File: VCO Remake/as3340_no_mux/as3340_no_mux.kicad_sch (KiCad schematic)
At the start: 83 parts, among them J1 Sync INput, J10 Conn_01x01_Male, J11 Conn_02x05_Odd_Even, J12 TRI OUt, J13 SIN OUT, J14 SAW OUt, J15 SQR OUT, J16 Conn_01x01_Male, J17 Conn_01x01_Male, J18 Conn_01x01_Male, J19 Conn_01x01_Male, J2 CV1, J20 Conn_01x01_Male, J21 Conn_01x01_Male, J22 Conn_01x06_Female, J23 Conn_01x06_Male, J24 Conn_01x01_Male, J25 Conn_01x01_Male, J26 Conn_01x01_Male, J27 Conn_01x01_Male, J28 Conn_01x01_Male, J29 Conn_01x01_Male, J3 Conn_01x01_Male, J30 Conn_01x01_Male, J4 LinearFmINput, J5 PWM INput, J6 Conn_01x01_Male, J7 Conn_01x01_Male, J8 Conn_01x01_Male, J9 Conn_01x01_Male, SW1 SW_SPDT, U1 LM13700, U2 AS3340, U4 LM324

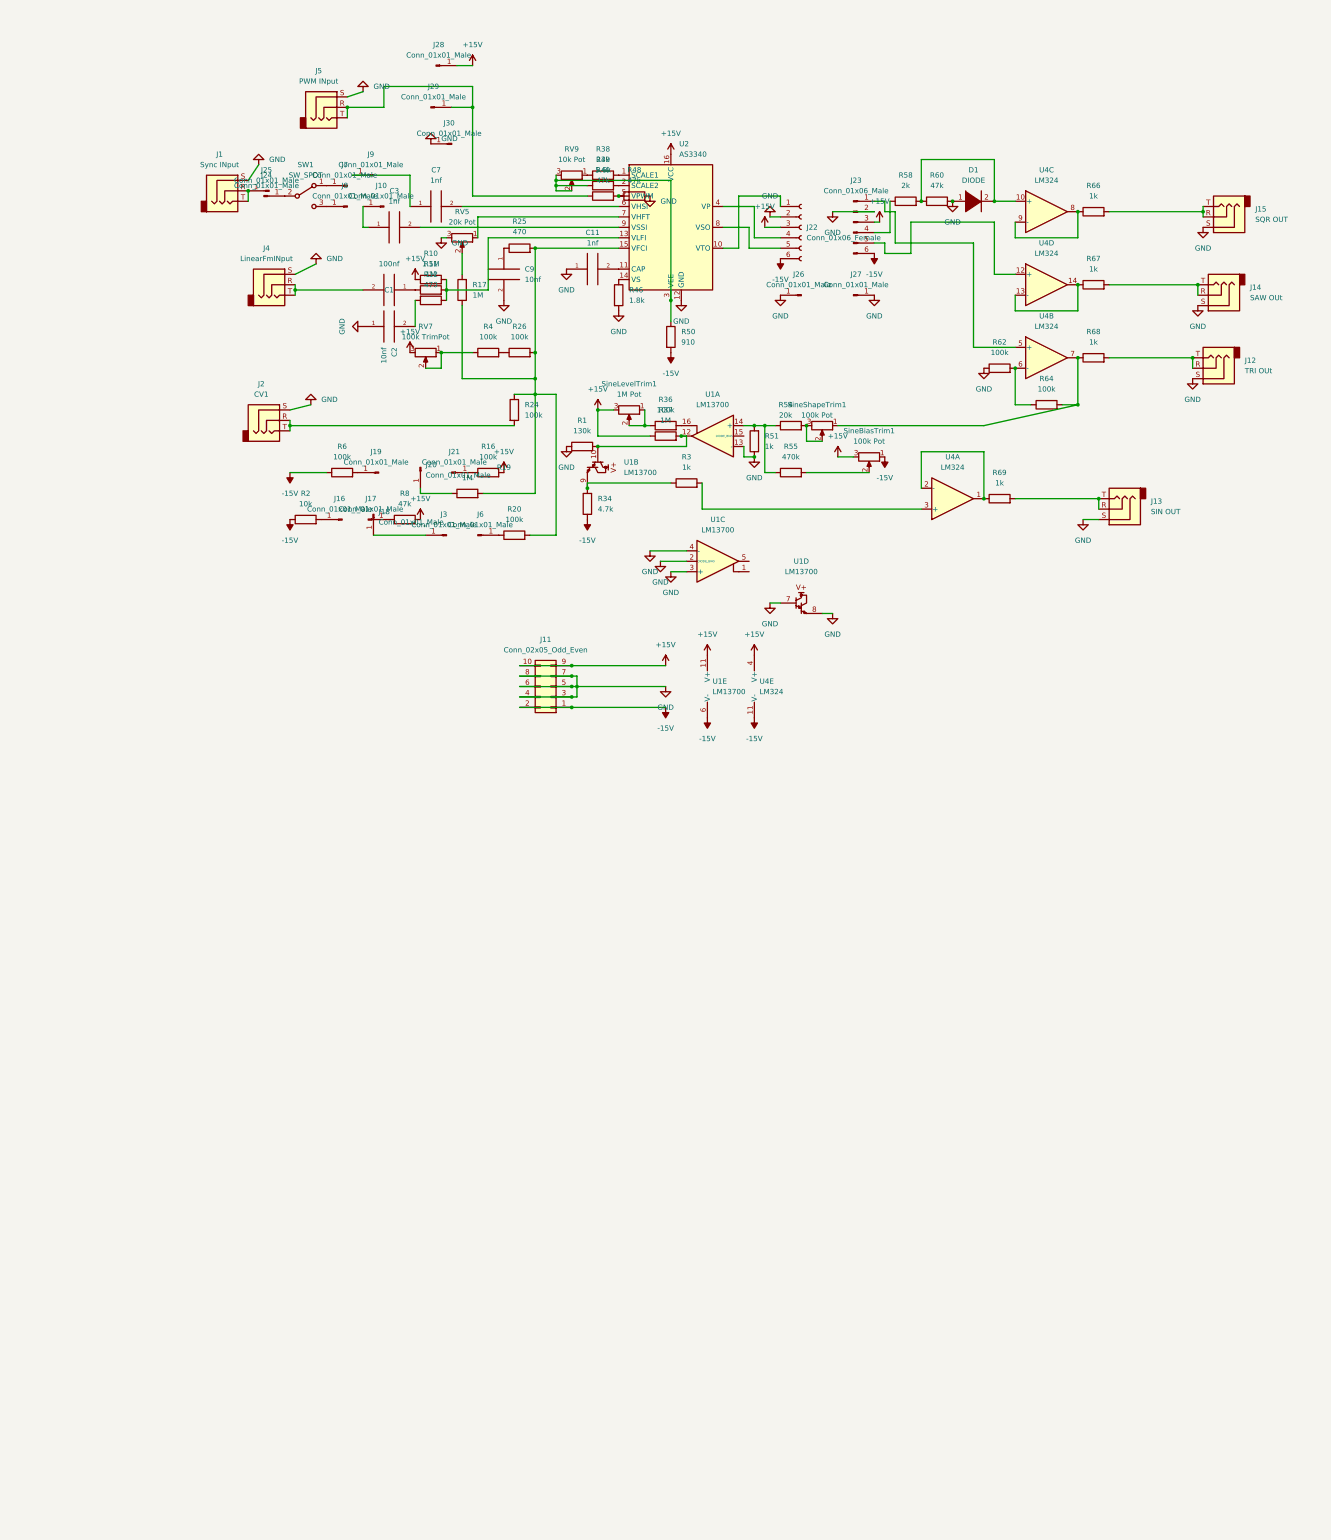
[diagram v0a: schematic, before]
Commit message: made schematic goof
not it good
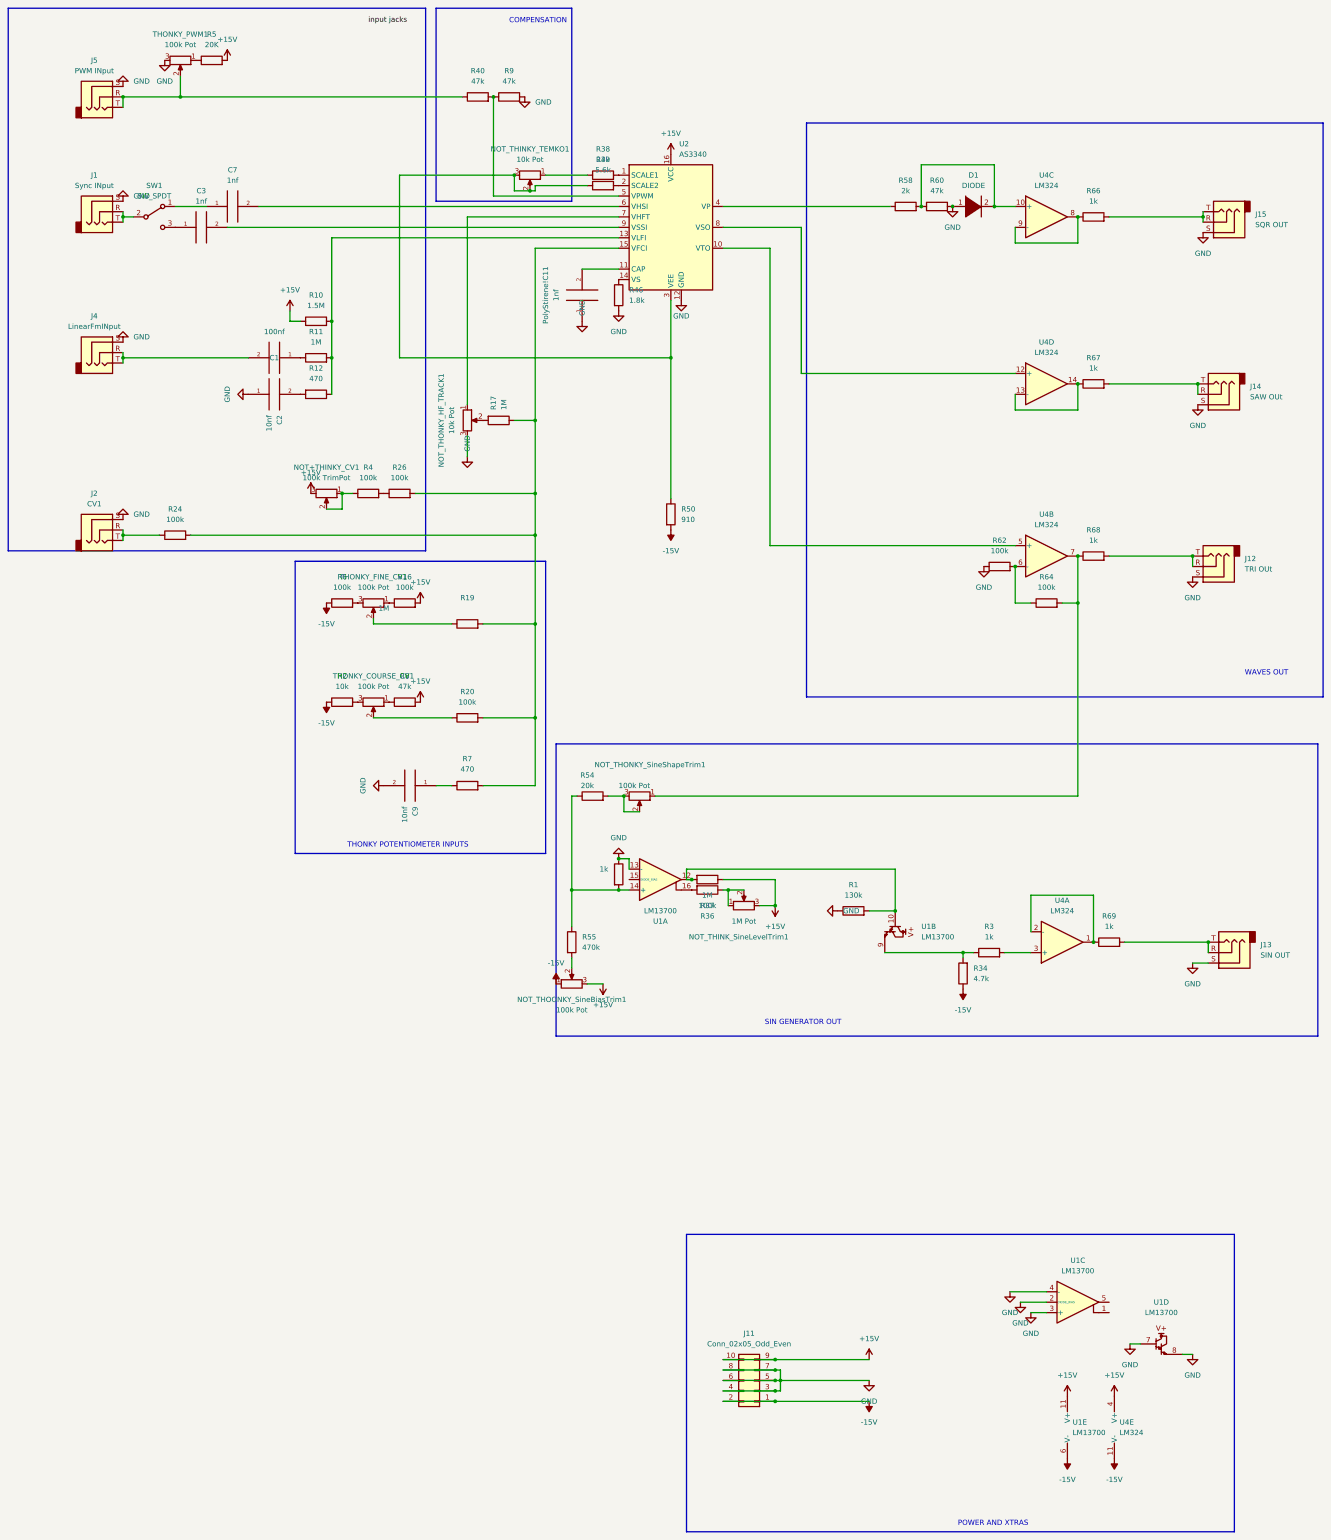
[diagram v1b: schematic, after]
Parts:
- removed J10, J16, J17, J18, J19, J20, J21, J24, J25, J26, J27, J28, J29, J3, J30, J6, J7, J8, J9: Conn_01x01_Male, Connector_PinHeader_2.54mm:PinHeader_1x01_P2.54mm_Vertical, symbol Connector:Conn_01x01_Male
- removed J22: Conn_01x06_Female, Connector_PinHeader_2.54mm:PinHeader_1x06_P2.54mm_Vertical, symbol Connector:Conn_01x06_Female
- removed J23: Conn_01x06_Male, Connector_PinHeader_2.54mm:PinHeader_1x06_P2.54mm_Vertical, symbol Connector:Conn_01x06_Male
- removed R25: 470, Resistor_SMD:R_1206_3216Metric, symbol Device:R
- removed R48: 47k, Resistor_SMD:R_1206_3216Metric, symbol Device:R
- added R5: 20K, Resistor_SMD:R_1206_3216Metric, symbol Device:R
- added R7: 470, Resistor_SMD:R_1206_3216Metric, symbol Device:R
- added R9: 47k, Resistor_SMD:R_1206_3216Metric, symbol Device:R
- added THONKY_COURSE_CV1, THONKY_FINE_CV1, THONKY_PWM1: 100k Pot, Potentiometer_THT:Potentiometer_Alps_RK09K_Single_Vertical, symbol Device:R_Potentiometer
- NOT_THONKY_HF_TRACK1: renamed from RV5; value 20k Pot -> 10k Pot
- renumbered RV7 to NOT+THINKY_CV1, RV9 to NOT_THINKY_TEMKO1, SineLevelTrim1 to NOT_THINK_SineLevelTrim1, SineShapeTrim1 to NOT_THONKY_SineShapeTrim1, SineBiasTrim1 to NOT_THOONKY_SineBiasTrim1, C11 to PolyStirene!C11
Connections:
- net +15V: now also R5.2
- net GND: now also R9.2, THONKY_PWM1.3
- net at J2.R, J2.T: now also R24.1; no longer R24.2
- net at U4.12 (+): now also U2.8 (VSO)
- net at J5.R, J5.T, R40.1: now also THONKY_PWM1.2
- net at R17.1, R19.2, R20.2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: now also R24.2, R7.2; no longer R24.1
- net at R20.1: now also THONKY_COURSE_CV1.2
- net at U2.10 (VTO): now also U4.5 (+)
- net at U2.4 (VP): now also R58.1
- net at R40.2, U2.5 (VPWM): now also R9.1
- net at R19.1: now also THONKY_FINE_CV1.2
- net at SW1.2 (B): now also J1.R, J1.T
- net at C9.1: now also R7.1
- net at C7.1: now also SW1.1 (A)
- net at R8.1: now also THONKY_COURSE_CV1.1
- net at SW1.3 (C): now also C3.1
- net at R2.2: now also THONKY_COURSE_CV1.3
- net at R16.1: now also THONKY_FINE_CV1.1
- net at R6.2: now also THONKY_FINE_CV1.3
- new net: R5.1, THONKY_PWM1.1
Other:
- note added: "COMPENSATION"
- note added: "POWER AND XTRAS"
- note added: "SIN GENERATOR OUT"
- note added: "THONKY POTENTIOMETER INPUTS"
- note added: "WAVES OUT"
- moved on the sheet: C1, C2, C3, C7, C9, D1, J1, J11, J12, J13, J14, J15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

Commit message: Very Epic 2 layer VCO
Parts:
- NOT+THINKY_CV1, NOT_THINKY_TEMKO1, NOT_THONKY_HF_TRACK1: footprint Potentiometer_THT:Potentiometer_Alps_RK09K_Single_Vertical -> Potentiometer_THT:Potentiometer_ACP_CA6-H2,5_Horizontal
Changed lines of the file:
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@@
       (effects (font (size 1.27 1.27)))
     )
-    (property "Footprint" "Potentiometer_THT:Potentiometer_Alps_RK09K_Single_Vertical" (at 167.64 138.43 0)
+    (property "Footprint" "Potentiometer_THT:Potentiometer_ACP_CA6-H2,5_Horizontal" (at 167.64 138.43 0)
       (effects (font (size 1.27 1.27)) hide)
     )
@@
       (effects (font (size 1.27 1.27)))
     )
-    (property "Footprint" "Potentiometer_THT:Potentiometer_Alps_RK09K_Single_Vertical" (at 201.93 120.65 0)
+    (property "Footprint" "Potentiometer_THT:Potentiometer_ACP_CA6-H2,5_Horizontal" (at 201.93 120.65 0)
       (effects (font (size 1.27 1.27)) hide)
     )
@@
       (effects (font (size 1.27 1.27)))
     )
-    (property "Footprint" "Potentiometer_THT:Potentiometer_Alps_RK09K_Single_Vertical" (at 217.17 60.96 0)
-      (effects (font (size 1.27 1.27)) hide)
-    )
+    (property "Footprint" "Potentiometer_THT:Potentiometer_ACP_CA6-H2,5_Horizontal" (at 217.17 60.96 0)
+      (effects (font (size 1.27 1.27)) hide)
+    )

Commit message: How????
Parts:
- PolyStirene!C11: footprint Capacitor_SMD:C_1206_3216Metric -> Capacitor_THT:C_Radial_D5.0mm_H5.0mm_P2.00mm
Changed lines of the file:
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@@
       (effects (font (size 1.27 1.27)))
     )
-    (property "Footprint" "Capacitor_SMD:C_1206_3216Metric" (at 229.87 90.17 0)
+    (property "Footprint" "Capacitor_THT:C_Radial_D5.0mm_H5.0mm_P2.00mm" (at 229.87 90.17 0)
       (effects (font (size 1.27 1.27)) hide)
     )

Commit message: Redone VCO Layout
Added the switch and made trace width .2mm
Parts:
- SW1: footprint Potentiometer_THT:Potentiometer_ACP_CA6-H2,5_Horizontal -> AAA MY Parts:Dailywell mini DWB1 SPDT
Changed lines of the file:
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@@
       (effects (font (size 1.27 1.27)))
     )
-    (property "Footprint" "Potentiometer_THT:Potentiometer_ACP_CA6-H2,5_Horizontal" (at 125.73 71.12 0)
+    (property "Footprint" "AAA MY Parts:Dailywell mini DWB1 SPDT" (at 125.73 71.12 0)
       (effects (font (size 1.27 1.27)) hide)
     )
